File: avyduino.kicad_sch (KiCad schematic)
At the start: 34 parts, among them J1 Power, J2 Digital/PWM, J3 Analog, J4 Digital/PWM, J5 USB_C_Receptacle_USB2.0_14P, Q1 AO3401A, U1 ATmega328P-P, U2 CH340G, U3 LM2931AZ-5.0_TO92, U4 MCP1700x-330xxTT, U5 LM358, Y1 12MHz, Y2 16MHz

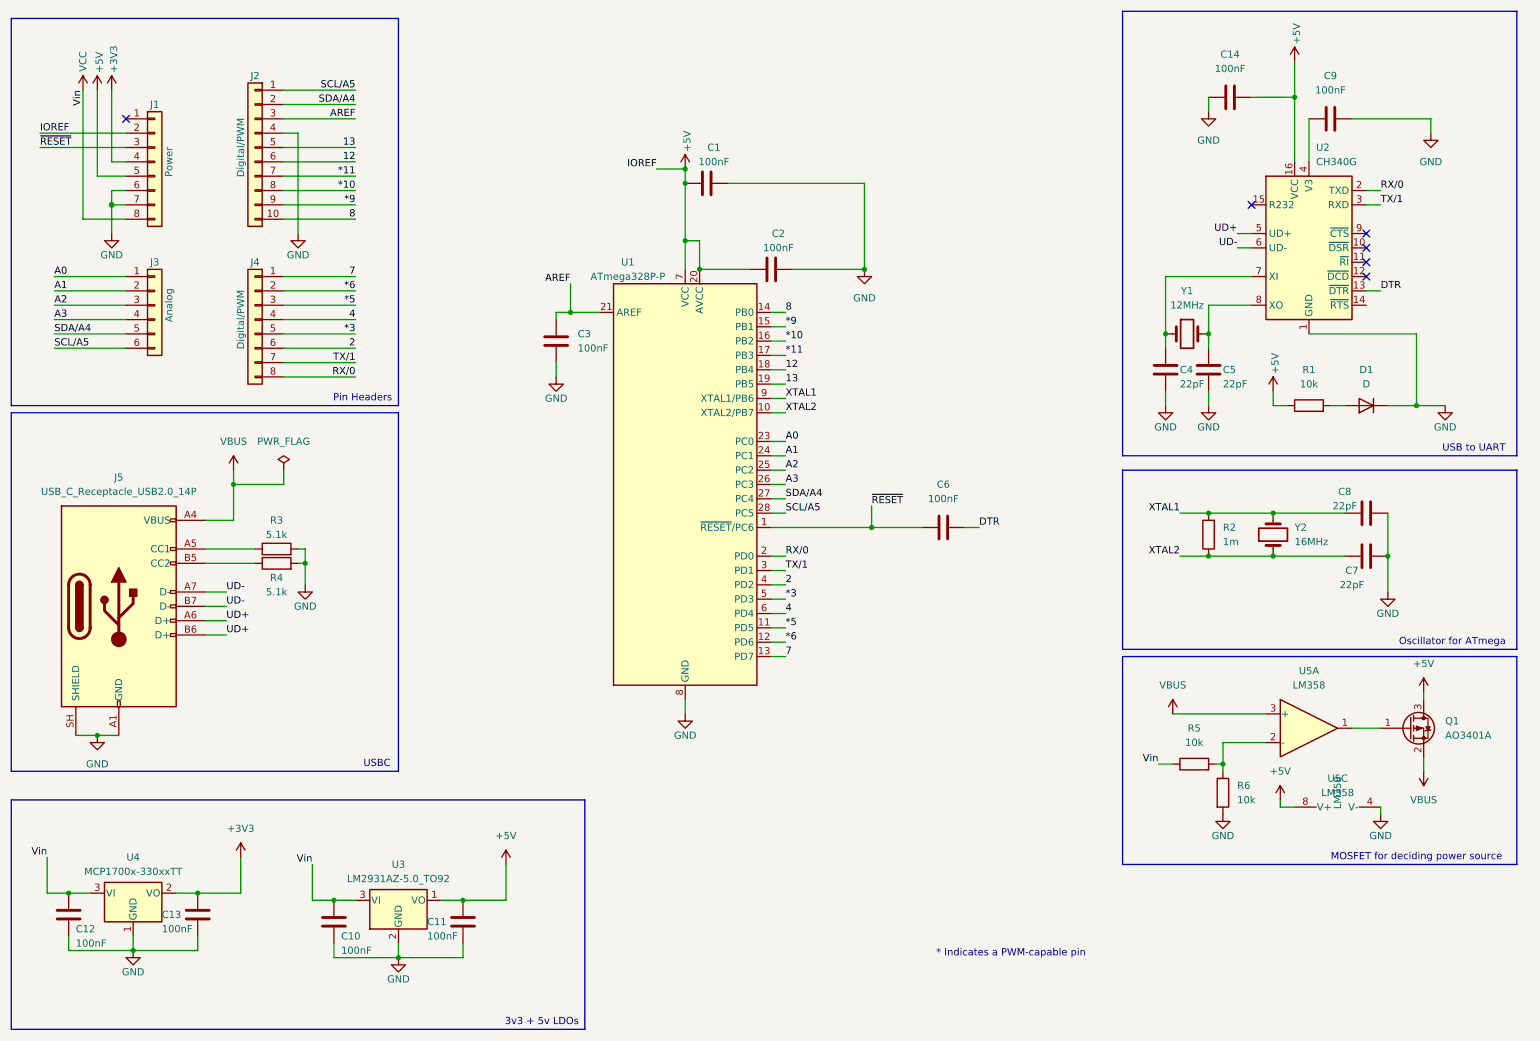
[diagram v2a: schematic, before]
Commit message: added icsp header
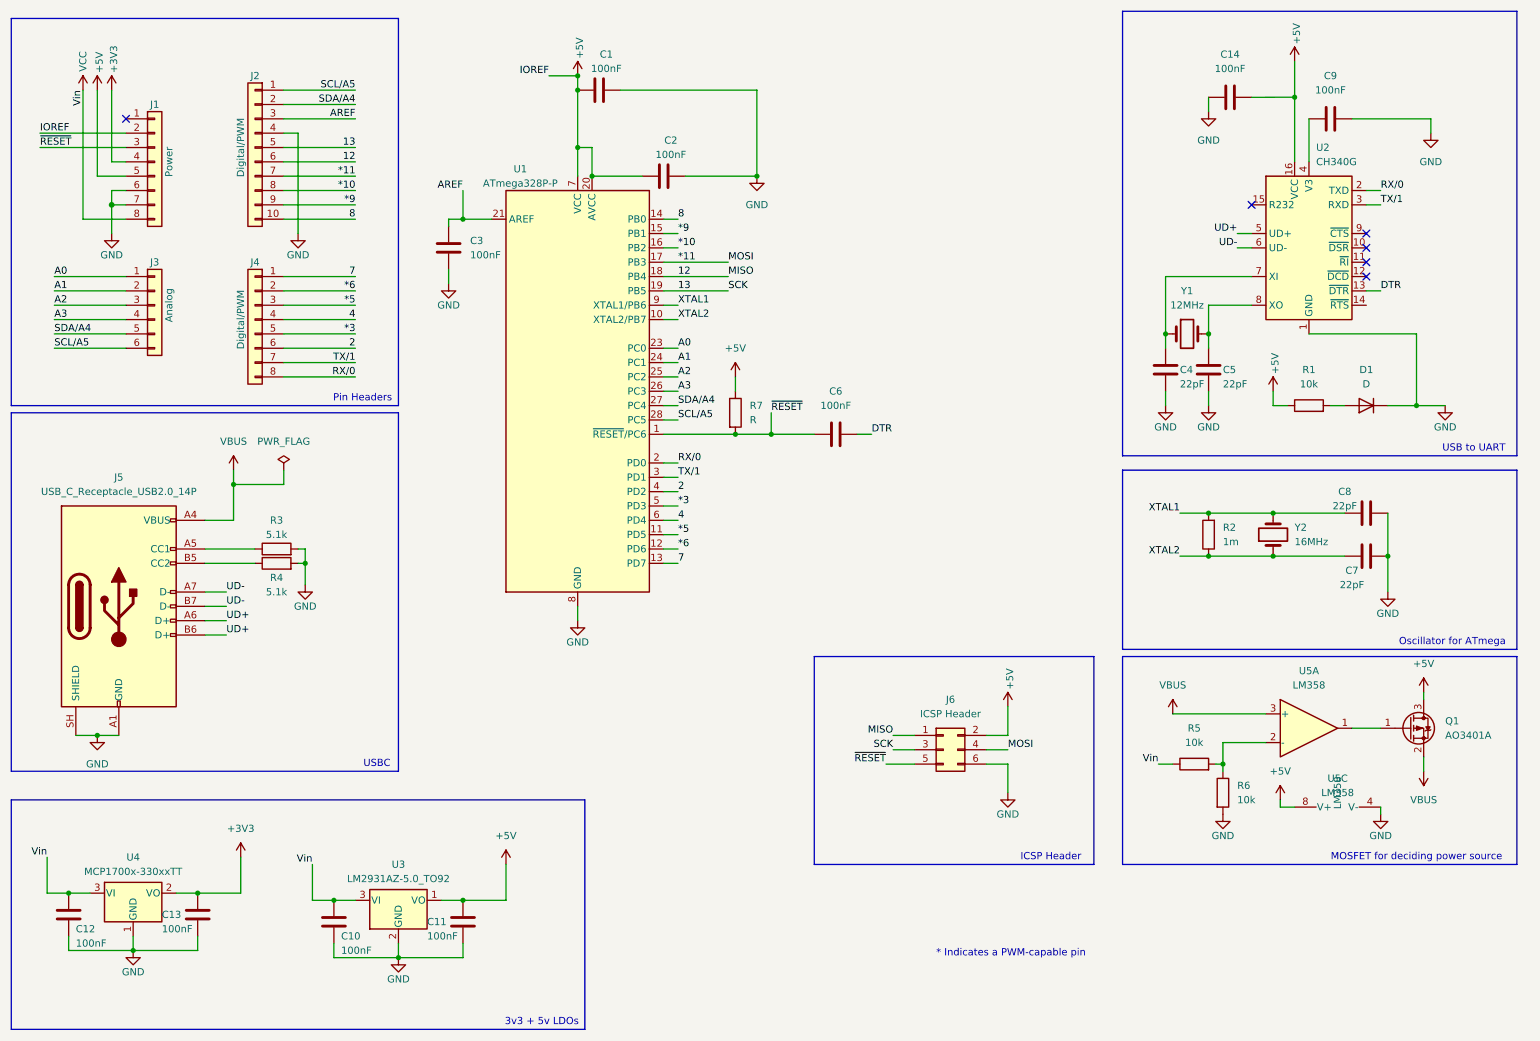
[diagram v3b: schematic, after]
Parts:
- added J6: ICSP Header, Connector_PinHeader_2.54mm:PinHeader_2x03_P2.54mm_Vertical, symbol Connector_Generic:Conn_02x03_Odd_Even
- added R7: R, Resistor_SMD:R_0805_2012Metric_Pad1.20x1.40mm_HandSolder, symbol Device:R
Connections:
- net *11: now also J6.4 (Pin_4)
- net +5V: now also J6.2 (Pin_2), R7.1
- net 12: now also J6.1 (Pin_1)
- net 13: now also J6.3 (Pin_3)
- net GND: now also J6.6 (Pin_6)
- net ~{RESET}: now also J6.5 (Pin_5), R7.2
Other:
- note added: "ICSP Header"
- moved on the sheet: C1, C2, C3, C6, U1
